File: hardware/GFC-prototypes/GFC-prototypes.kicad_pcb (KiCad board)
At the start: 2 copper layers, 11.2 x 14.2 mm, 6 parts, among them J1 Conn_01x05_Male, U1 BME280

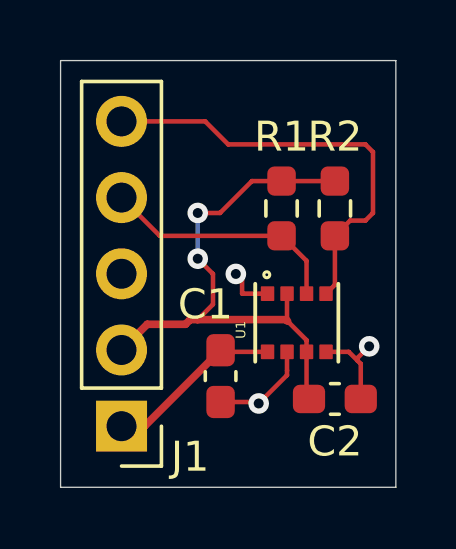
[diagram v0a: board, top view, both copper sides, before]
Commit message: PCB Prototype
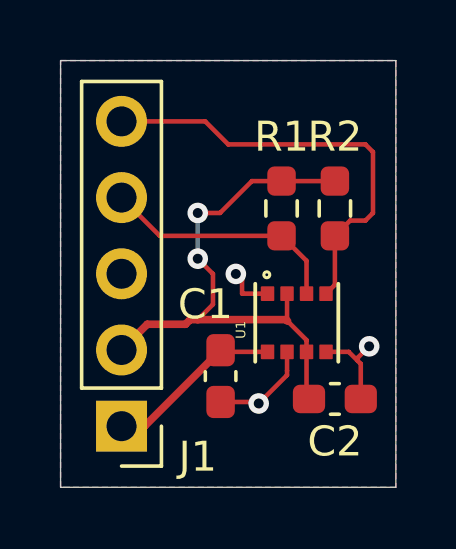
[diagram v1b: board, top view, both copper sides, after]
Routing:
- added copper zone on B.Cu, net GND
- added copper zone on F.Cu, net GND
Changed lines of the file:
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@@
     (property "Sheetname" "")
     (attr through_hole)
-    (fp_text reference "J1" (at -2.286 -1.021 180) (layer "F.SilkS")
+    (fp_text reference "J1" (at -2.54 -1.021 180) (layer "F.SilkS")
       (effects (font (size 1 1) (thickness 0.15)))
     )
@@
   (segment (start 72.903 33.274) (end 71.628 31.999) (width 0.1524) (layer "F.Cu") (net 5))
   (segment (start 77.795 34.107) (end 76.962 33.274) (width 0.1524) (layer "F.Cu") (net 5))
+  (zone (net 1) (net_name "GND") (layers F&B.Cu) (hatch edge 0.508)
+    (connect_pads (clearance 0.508))
+    (min_thickness 0.254) (filled_areas_thickness no)
+    (fill yes (thermal_gap 0.508) (thermal_bridge_width 0.508))
+    (polygon
+      (pts
+        (xy 80.772 41.656)
+        (xy 69.596 41.656)
+        (xy 69.596 27.432)
+        (xy 80.772 27.432)
+      )
+    )
+  )
 )
